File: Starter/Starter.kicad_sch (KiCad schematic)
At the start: 64 parts, among them J2 Speaker, J3 UART1, J5 Conn_01x08_Pin, M1 Vibration Motor, Q1 2N2222, SW1 UP, SW2 LEFT, SW3 DOWN, SW4 RIGHT, U1 MPU-6050, U2 LP-MSPM0G3507, U3 MCP34119D, U4 HiLetGo_ST7735R, U5 ULN2003B, U6 TSOP31438

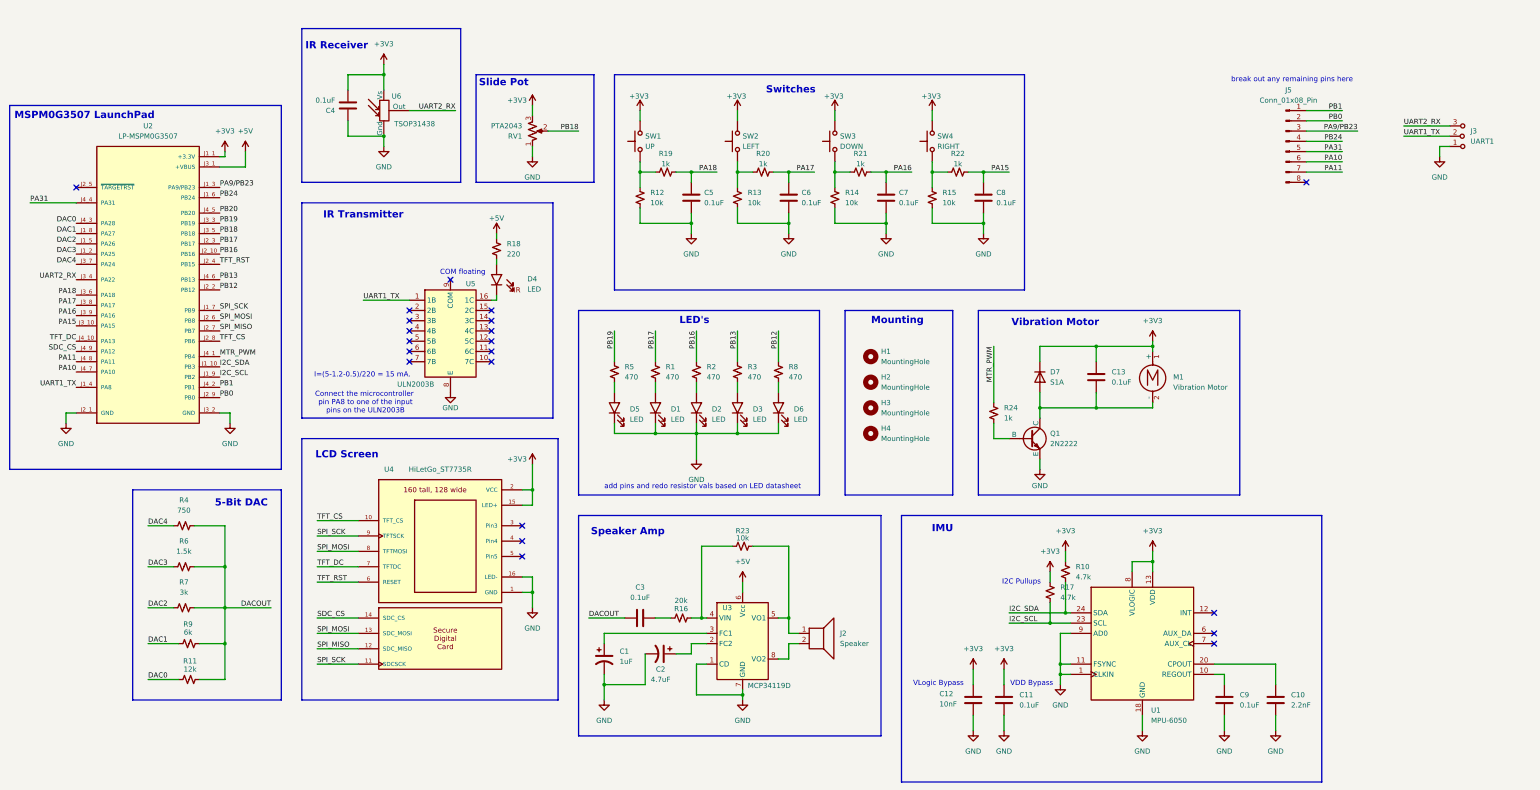
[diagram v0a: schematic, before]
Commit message: structure changes
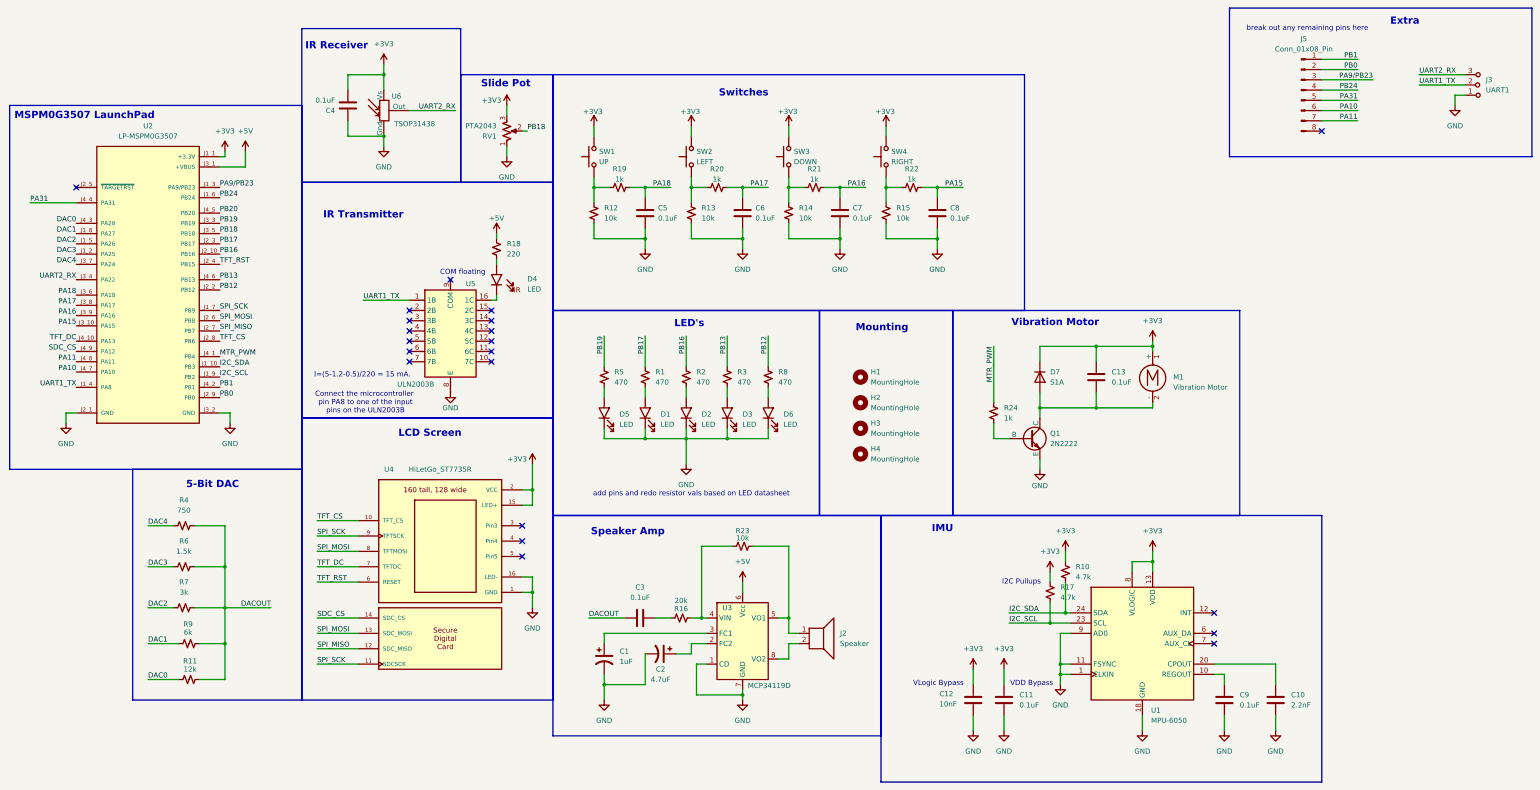
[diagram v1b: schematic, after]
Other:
- note added: "Extra"
- moved on the sheet: C5, C6, C7, C8, D1, D2, D3, D5, D6, H1, H2, H3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
